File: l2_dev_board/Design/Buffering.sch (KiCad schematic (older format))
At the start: 20 parts, among them U302 NC7WZ17, U303 NC7WZ17, U304 NC7WZ17, U305 NC7WZ17, U306 NC7WZ17, U307 NC7WZ17, U308 NC7WZ17, U309 NC7WZ17, U310 NC7WZ17, U311 NC7WZ17

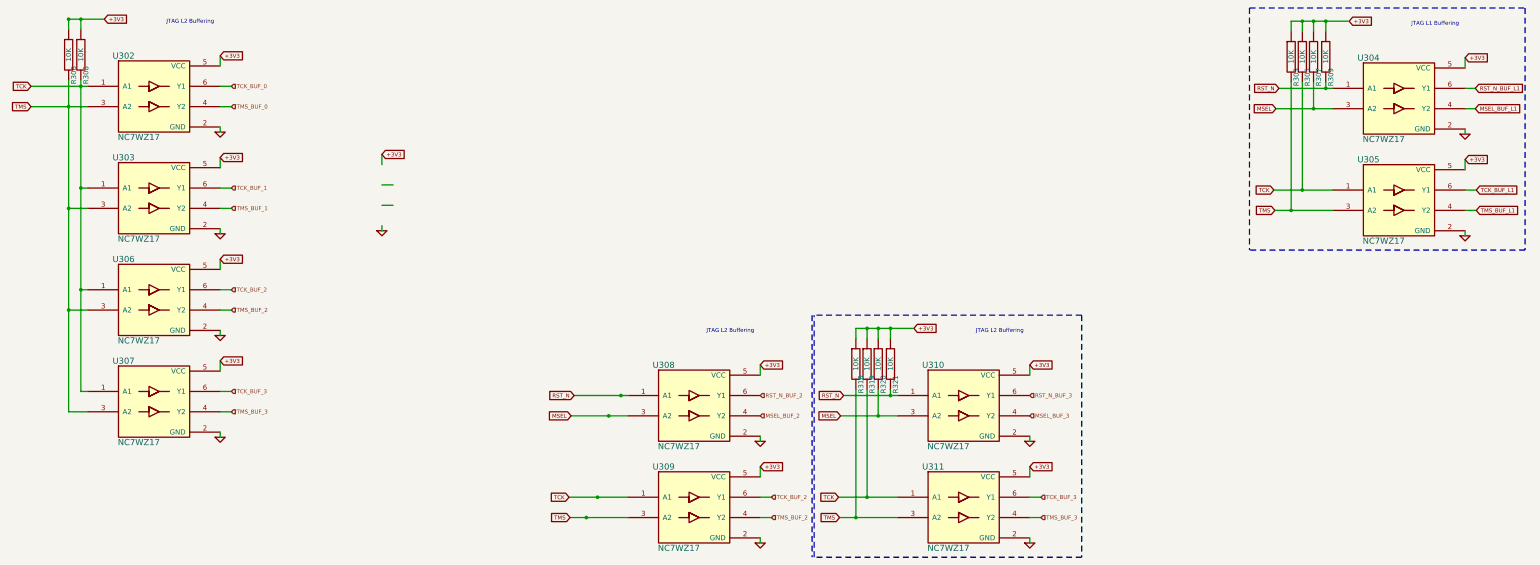
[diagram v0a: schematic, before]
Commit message: Isolated L1 stuff (inc. JTAG) in single sheet. Added buffered for the L2's JTAG control signals.
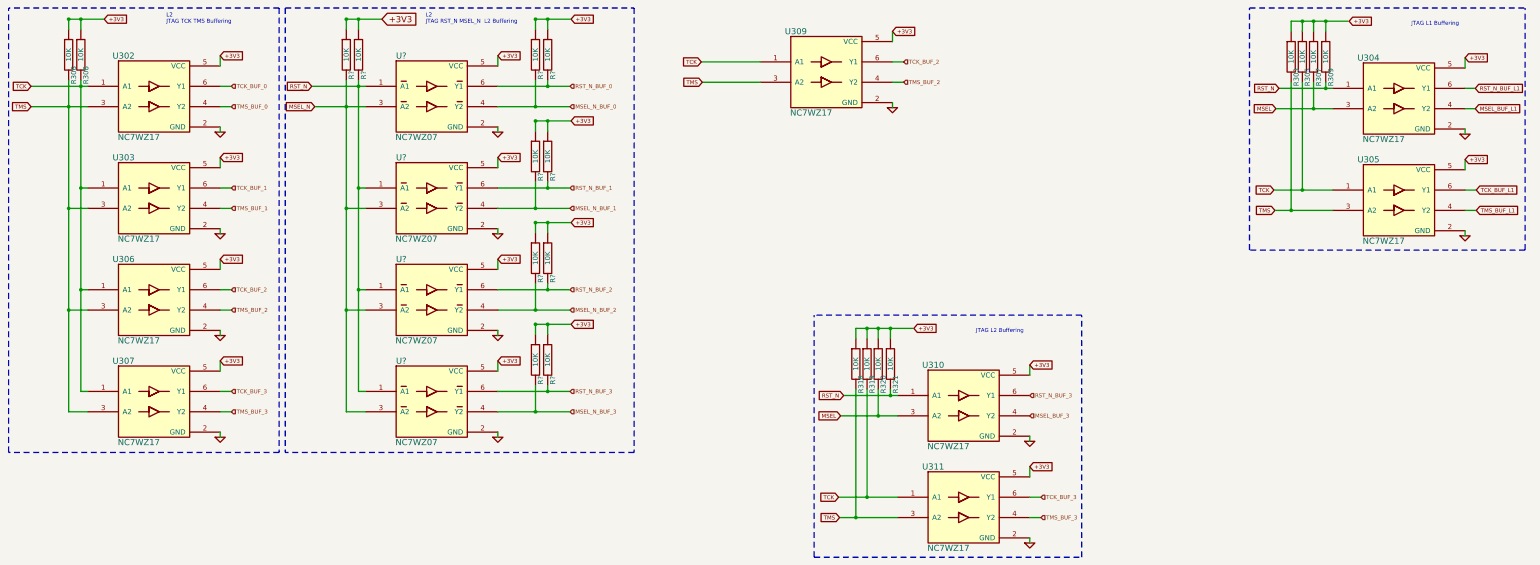
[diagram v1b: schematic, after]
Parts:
- removed U308: NC7WZ17, symbol NC7WZ17
- added R? (x10): 10K, symbol R
- added U? (x4): NC7WZ07, symbol NC7WZ07
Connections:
- net labels added: MSEL_N, MSEL_N_BUF_0, MSEL_N_BUF_1, MSEL_N_BUF_2, MSEL_N_BUF_3, RST_N_BUF_0, RST_N_BUF_1
- net labels removed: MSEL_BUF_2
- wire segments 113 -> 125
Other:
- note added: "L2 \nJTAG TCK TMS Buffering"
- note added: "L2\nJTAG RST_N MSEL_N L2 Buffering"
- moved on the sheet: U309
